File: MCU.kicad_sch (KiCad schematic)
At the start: 14 parts, among them J2 FTDI, SW1 SW_MEC_5G, SW2 SW_MEC_5G, U1 ESP32-WROOM-32, U5 PCF8574

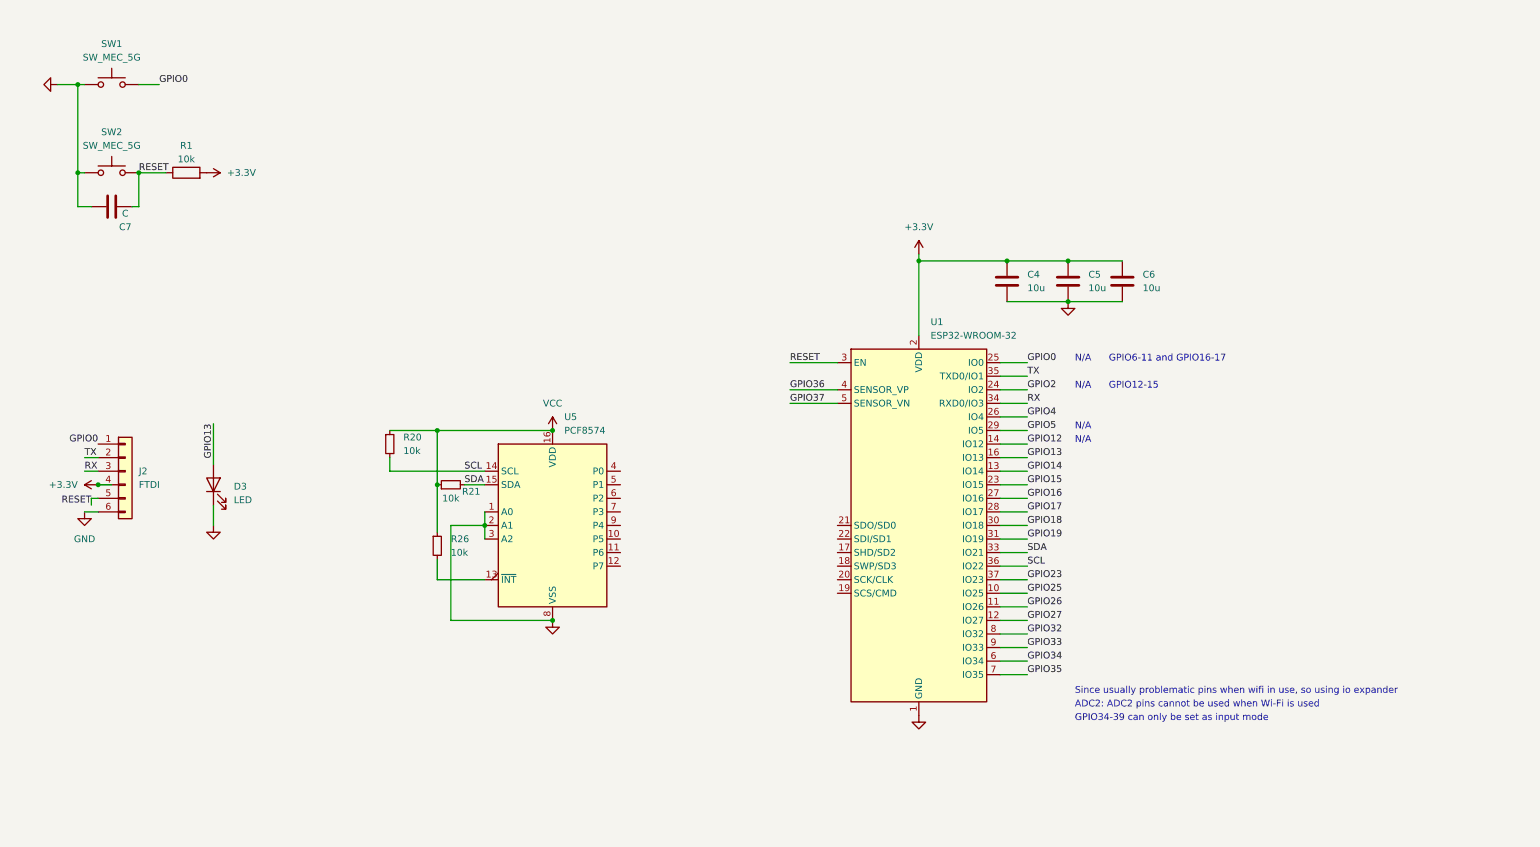
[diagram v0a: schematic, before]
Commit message: Schematic Completed
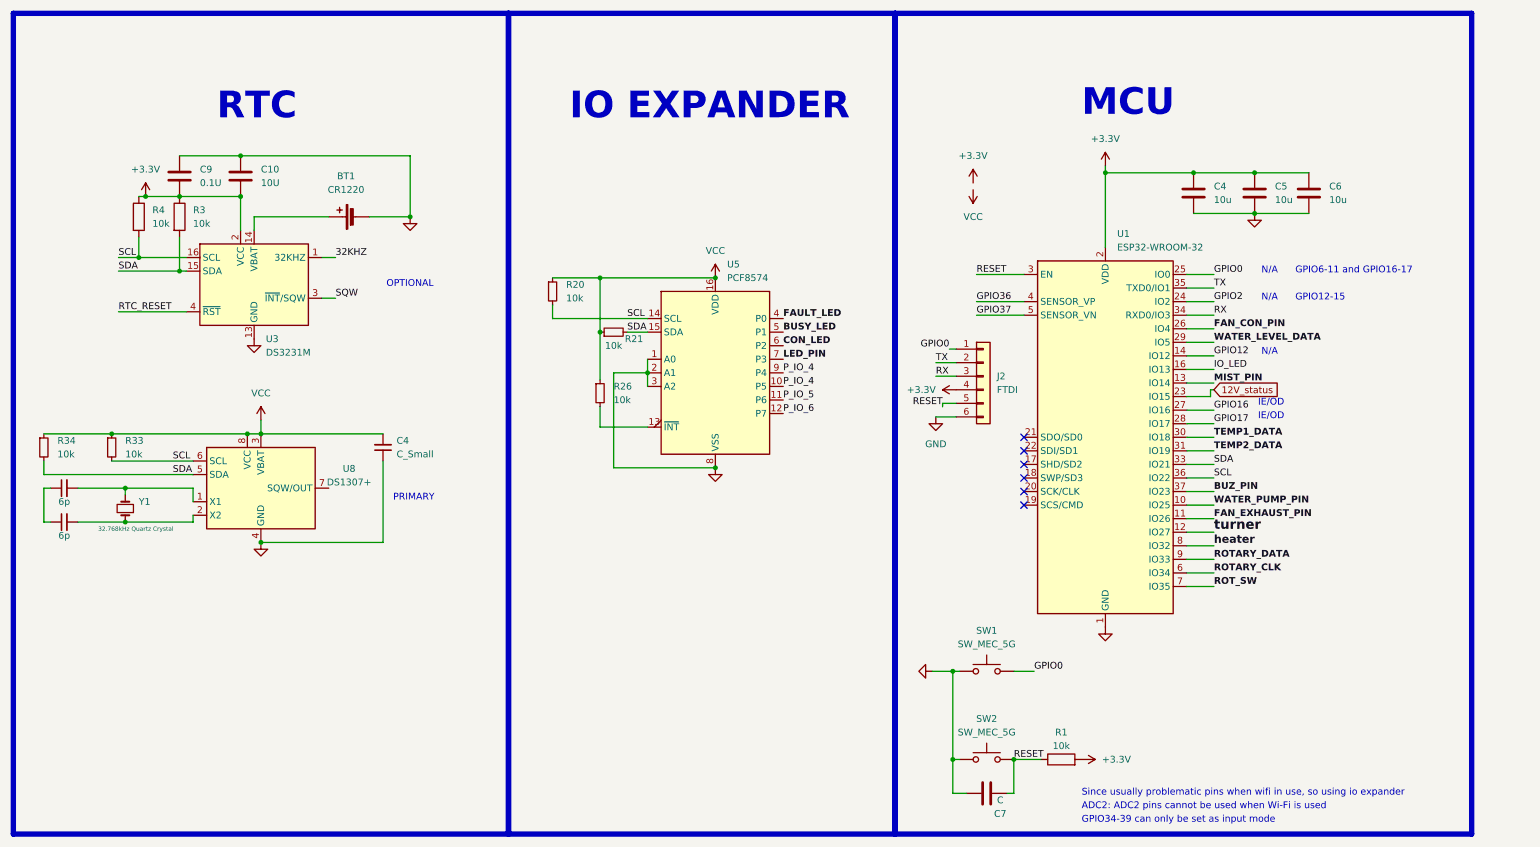
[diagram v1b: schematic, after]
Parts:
- removed D3: LED, symbol Device:LED
- added BT1: CR1220, symbol Device:Battery_Cell
- added C10: 10U, symbol Device:C
- added C11, C12: 6p, symbol Device:C_Small
- added C4: C_Small, symbol Device:C_Small
- added C9: 0.1U, symbol Device:C
- added R3, R4: 10k, symbol Device:R
- added R33, R34: 10k, symbol Device:R_Small
- added U3: DS3231M, Package_SO:SOIC-16W_7.5x10.3mm_P1.27mm, symbol Timer_RTC:DS3231M
- added U8: DS1307+, Package_DIP:DIP-8_W7.62mm, symbol Timer_RTC:DS1307+
- added Y1: 32.768kHz Quartz Crystal, symbol Device:Crystal_Small
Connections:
- net +3.3V: now also C10.1, C9.1, R3.1, R4.1, U3.2 (VCC)
- net GND: now also BT1.2 (-), C10.2, C4.1, C9.2, U3.10 (GND), U3.11 (GND), U3.12 (GND), U3.13 (GND), U3.5 (GND), U3.6 (GND), U3.7 (GND), U3.8 (GND), U3.9 (GND), U8.4 (GND)
- net SCL: now also R33.2, R4.2, U3.16 (SCL), U8.6 (SCL)
- net SDA: now also R3.2, R34.2, U3.15 (SDA), U8.5 (SDA)
- net VCC: now also C4.2, R33.1, R34.1, U8.3 (VBAT), U8.8 (VCC)
- net P_IO_4: now reaches U5.10 (P5)
- net P_IO_4: now also U5.9 (P4)
- net P_IO_5: now reaches U5.11 (P6)
- net P_IO_6: now reaches U5.12 (P7)
- net FAULT_LED: now reaches U5.4 (P0)
- net BUSY_LED: now reaches U5.5 (P1)
- net CON_LED: now reaches U5.6 (P2)
- net LED_PIN: now reaches U5.7 (P3)
- net GPIO13 renamed IO_LED
- net GPIO14 renamed MIST_PIN
- net GPIO15 renamed 12V_status
- net GPIO18 renamed TEMP1_DATA
- net GPIO19 renamed TEMP2_DATA
- net GPIO23 renamed BUZ_PIN
- net GPIO25 renamed WATER_PUMP_PIN
- net GPIO26 renamed FAN_EXHAUST_PIN
- net GPIO27 renamed turner
- net GPIO32 renamed heater
- net GPIO33 renamed ROTARY_DATA
- net GPIO34 renamed ROTARY_CLK
- net GPIO35 renamed ROT_SW
- net GPIO4 renamed FAN_CON_PIN
- net GPIO5 renamed WATER_LEVEL_DATA
- new net: BT1.1 (+), U3.14 (VBAT)
- new net: C11.1, C12.1
- new net: C12.2, U8.1 (X1), Y1.2
- new net: C11.2, U8.2 (X2), Y1.1
- new net 32KHZ: U3.1 (32KHZ)
- new net RTC_RESET: U3.4 (~{RST})
- new net SQW: U3.3 (~{INT}/SQW)
- no-connect marks 0 -> 6
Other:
- note added: "IE/OD"
- note added: "IO EXPANDER"
- note added: "MCU"
- note added: "OPTIONAL"
- note added: "PRIMARY"
- note added: "RTC"
- moved on the sheet: C4, C5, C6, C7, J2, R1, R20, R21, R26, SW1, SW2, U1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
